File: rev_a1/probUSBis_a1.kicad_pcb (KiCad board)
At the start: 2 copper layers, 44.5 x 22.9 mm, 26 parts, among them CON1 USB-MINI-B, IC1 ATTINY85-P, P1 USB_A_MALE, P2 CONN_8, P3 CONN_4, U1 LM78L05ACZ

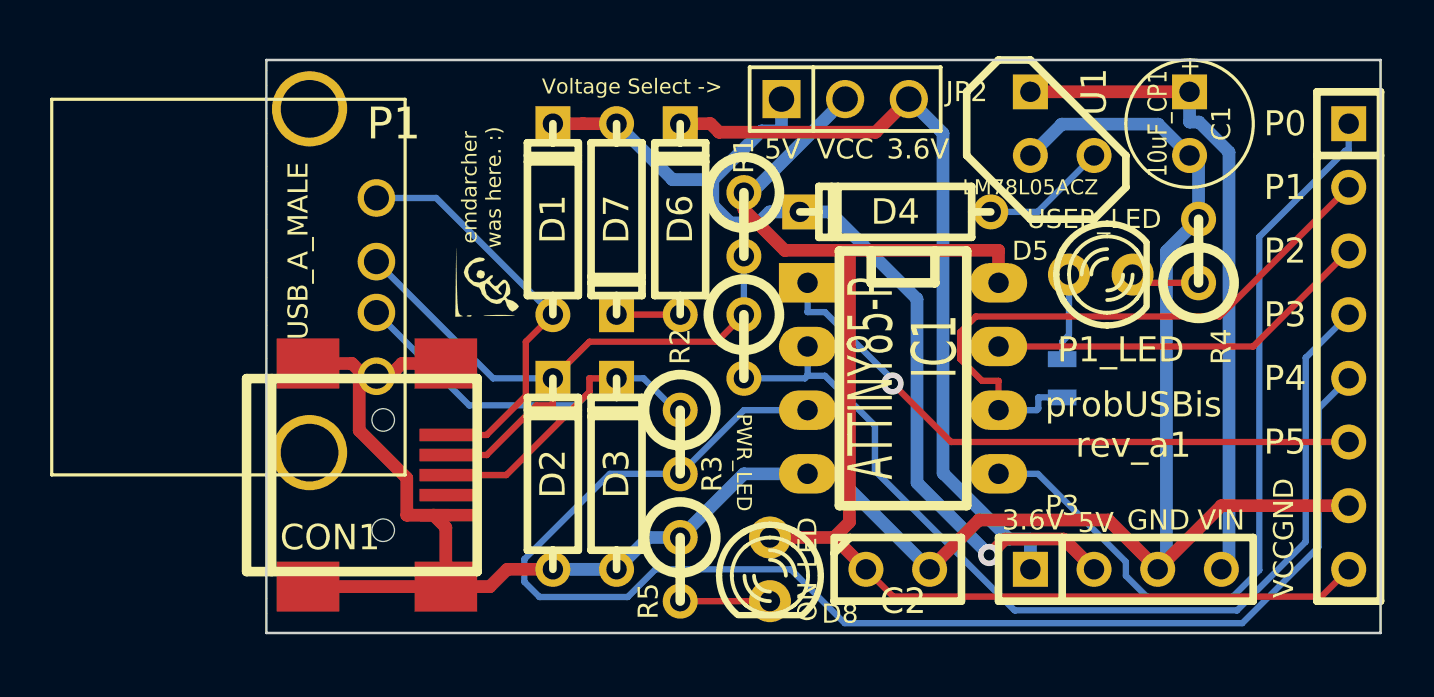
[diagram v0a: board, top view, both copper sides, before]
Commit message: generating files
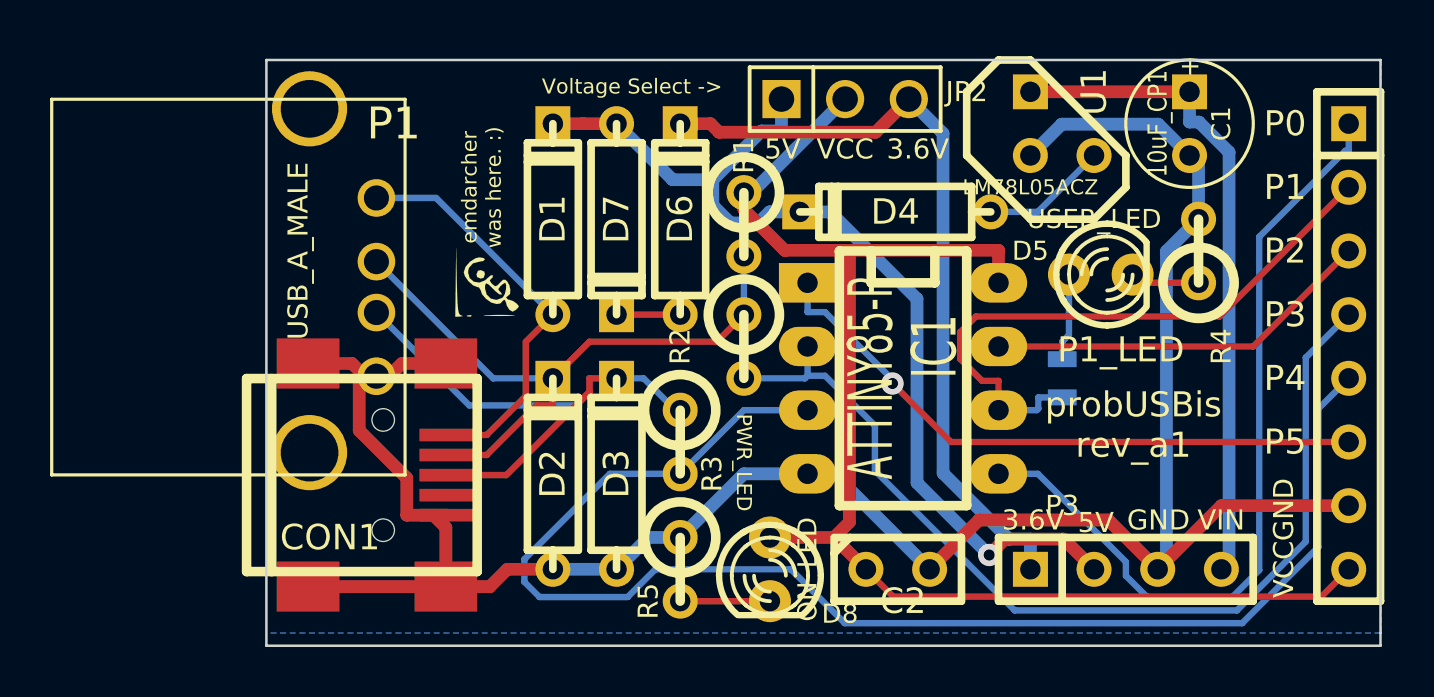
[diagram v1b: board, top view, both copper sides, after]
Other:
- board size 44.5 x 22.9 mm -> 44.5 x 23.4 mm
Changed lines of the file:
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@@
     (links 52)
     (no_connects 1)
-    (area 96.528499 90.0028 152.40127 114.59845)
+    (area 96.528499 90.0028 152.38476 114.929)
     (thickness 1.6)
-    (drawings 41)
+    (drawings 42)
     (tracks 183)
     (zones 0)
@@
   (page A4)
   (layers
-    (15 F.Cu signal hide)
-    (0 B.Cu signal hide)
+    (15 F.Cu signal)
+    (0 B.Cu signal)
     (16 B.Adhes user)
     (17 F.Adhes user)
@@
     (visible_elements FFFFFF7F)
     (pcbplotparams
-      (layerselection 3178497)
+      (layerselection 284196865)
       (usegerberextensions true)
       (excludeedgelayer true)
@@
       (xy 4.572 0.45466) (xy 4.572 0.46736) (xy 4.572 1.0922) (xy 4.572 1.0922)) (layer B.SilkS) (width 0.00254))
   )
+  (gr_line (start 149.86 114.808) (end 149.86 114.3) (angle 90) (layer Edge.Cuts) (width 0.1))
   (gr_text "Open Source\nHardware" (at 115.57 107.95 90) (layer B.SilkS)
     (effects (font (size 0.8 0.8) (thickness 0.2)) (justify mirror))
   )
-  (gr_line (start 105.41 114.3) (end 105.41 91.44) (angle 90) (layer Edge.Cuts) (width 0.1))
-  (gr_line (start 149.86 114.3) (end 105.41 114.3) (angle 90) (layer Edge.Cuts) (width 0.1))
+  (gr_line (start 105.41 114.808) (end 105.41 91.44) (angle 90) (layer Edge.Cuts) (width 0.1))
+  (gr_line (start 149.86 114.808) (end 105.41 114.808) (angle 90) (layer Edge.Cuts) (width 0.1))
   (gr_line (start 149.86 91.44) (end 149.86 114.3) (angle 90) (layer Edge.Cuts) (width 0.1))
   (gr_line (start 105.41 91.44) (end 149.86 91.44) (angle 90) (layer Edge.Cuts) (width 0.1))
